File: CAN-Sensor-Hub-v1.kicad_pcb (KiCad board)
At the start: 2 copper layers, 51 x 55 mm, 62 parts, among them J1 Conn_01x04, J10 Conn_01x03, J11 Conn_01x03, J2 Conn_01x04, J3 Conn_01x04, J4 USB_C_Receptacle_USB2.0_14P, J5 Conn_ARM_JTAG_SWD_10, J6 Conn_01x04, J7 Conn_01x04, J8 Conn_01x04, J9 Conn_01x03, Q1 NMOS, Q2 NMOS, Q3 PMOS, SW1 NRST, SW2 BOOT, U1 TPS5430DDA, U2 TCAN1042DRQ1, U3 W25Q32JVZP, U4 AZ1117-3.3, U7 STM32F722VETx, X1 8MHz, X2 32.768KHz

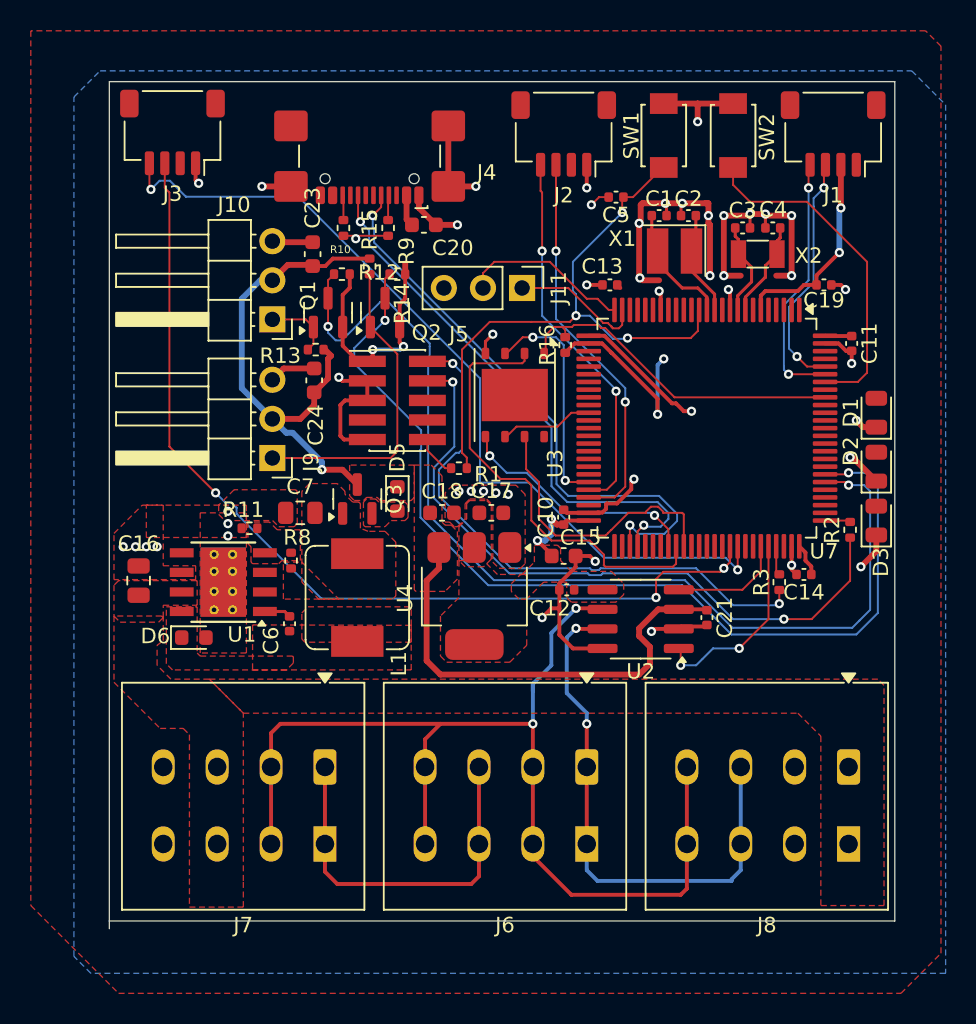
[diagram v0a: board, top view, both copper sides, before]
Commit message: V0.2 of board, nearly ready for production
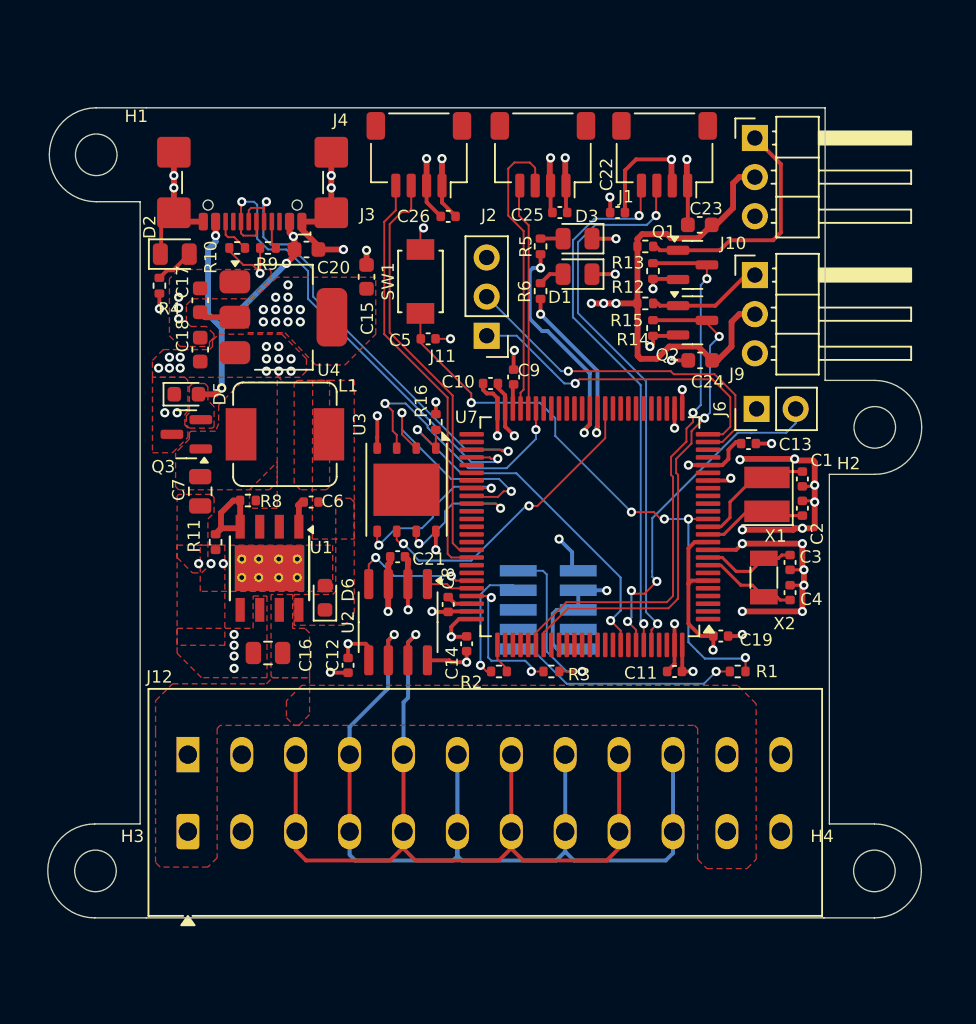
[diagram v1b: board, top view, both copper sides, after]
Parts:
- removed J7, J8: Conn_01x04, TerminalBlock_WAGO:TerminalBlock_WAGO_2601-1104_1x04_P3.50mm_Horizontal
- removed SW2: BOOT, lib:SW_TS-1088-AR02016
- added C22: 100nF, Capacitor_SMD:C_0402_1005Metric, F.Cu at (156.0, 67.5)
- added C25: 100nF, Capacitor_SMD:C_0402_1005Metric, F.Cu at (152.2, 67.5)
- added C26: 100nF, Capacitor_SMD:C_0402_1005Metric, F.Cu at (145.0, 67.8)
- added C8: 2.2uF, Capacitor_SMD:C_0402_1005Metric, F.Cu at (145.0, 93.0)
- added C9: 2.2uF, Capacitor_SMD:C_0402_1005Metric, F.Cu at (149.2, 78.2)
- added H1: MountingHole, MountingHole:MountingHole_2.7mm_M2.5, F.Cu at (122.2, 63.8)
- added H2: MountingHole, MountingHole:MountingHole_2.7mm_M2.5, F.Cu at (172.7, 81.5)
- added H3: MountingHole, MountingHole:MountingHole_2.7mm_M2.5, F.Cu at (122.1, 110.2)
- added H4: MountingHole, MountingHole:MountingHole_2.7mm_M2.5, F.Cu at (172.7, 110.2)
- added J12: Conn_01x12, TerminalBlock_WAGO:TerminalBlock_WAGO_2601-1112_1x12_P3.50mm_Horizontal, F.Cu at (128.1, 107.7)
- added R4: 160, Resistor_SMD:R_0402_1005Metric, F.Cu at (126.2, 72.2)
- added R5: 60, Resistor_SMD:R_0402_1005Metric, F.Cu at (151.0, 69.7)
- added R6: 160, Resistor_SMD:R_0402_1005Metric, F.Cu at (151.0, 72.6)
- J5: moved to B.Cu
- J6: value Conn_01x04 -> Conn_01x02; footprint TerminalBlock_WAGO:TerminalBlock_WAGO_2601-1104_1x04_P3.50mm_Horizontal -> Connector_PinHeader_2.54mm:PinHeader_1x02_P2.54mm_Vertical
- moved D2 47.6 mm to (127.2, 70.2), turned to 0 degrees
- moved J9 33.5 mm to (164.9, 71.6), turned to 0 degrees
- moved J10 33.5 mm to (164.9, 62.7), turned to 0 degrees
- moved D3 26.7 mm to (153.4, 69.2), turned to 180 degrees
- moved J6 25.7 mm to (165.0, 80.2), turned to 90 degrees
- moved C23 25.2 mm to (161.3, 68.3), turned to 180 degrees
- moved C24 25.1 mm to (161.4, 77.1), turned to 180 degrees
- moved R2 24.6 mm to (148.3, 97.3), turned to 0 degrees
- moved C11 24.2 mm to (159.7, 97.3), turned to 180 degrees
- moved Q1 23.9 mm to (160.9, 70.9), turned to 0 degrees
- moved C19 23.8 mm to (162.7, 95.0)
- moved C4 23.7 mm to (167.2, 92.2), turned to 90 degrees
- moved C17 23.4 mm to (128.9, 73.2), turned to 90 degrees
- moved R13 22.4 mm to (157.8, 69.7), turned to 0 degrees
- moved R1 22.4 mm to (163.8, 97.3)
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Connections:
- D1 pad 2: unconnected-(D1-A-Pad2) -> Net-(D1-A)
- D2 pad 2: unconnected-(D2-A-Pad2) -> Net-(D2-A)
- D3 pad 2: unconnected-(D3-A-Pad2) -> Net-(D3-A)
- J11 pad 1: USART2_TX -> USART2_RX
- J11 pad 2: USART2_RX -> USART2_TX
- J6 pad 1: CAN_H -> GNDREF
- J6 pad 2: CAN_L -> Net-(J6-Pin_2)
- U7 pad 37: unconnected-(U7-PE7-Pad37) -> IO_LED3
- U7 pad 38: unconnected-(U7-PE8-Pad38) -> IO_LED2
- U7 pad 39: unconnected-(U7-PE9-Pad39) -> IO_LED1
- U7 pad 48: unconnected-(U7-VCAP_1-Pad48) -> Net-(U7-VCAP_1)
- U7 pad 73: unconnected-(U7-VCAP_2-Pad73) -> Net-(U7-VCAP_2)
- U7 pad 94: Net-(U7-BOOT0) -> Net-(J6-Pin_2)
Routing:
- net Net-(J5-SWCLK/TCK): track 44.1 -> 8.29 mm, vias 2 -> 1
- net I2C3_SDA: track 61.9 -> 26.8 mm, vias 3 -> 0
- net DIO_1_3V3: track 64.2 -> 33.6 mm
- net DIO_0_3V3: track 67.2 -> 36.7 mm
- net I2C3_SCL: track 55.9 -> 27.2 mm, vias 2 -> 0
- net Net-(J5-SWDIO/TMS): track 37.4 -> 11.3 mm, vias 2 -> 1
- net VBUS_5V: track 2.06 -> 27.3 mm, vias 0 -> 4
- net Net-(J6-Pin_2): track 0.00 -> 22.9 mm, vias 0 -> 3
- net Net-(U7-BOOT0): track 22.1 -> 0.00 mm
- net I2C1_SDA: track 15.8 -> 35.9 mm
- net I2C1_SCL: track 16.7 -> 34.9 mm
- net IO_LED2: track 0.00 -> 15.9 mm, vias 0 -> 2
- net USART2_TX: track 8.70 -> 23.1 mm, vias 0 -> 1
- net QSPI_CLK: track 5.98 -> 19.9 mm, vias 0 -> 2
- net QSPI_IO1: track 29.2 -> 15.3 mm, vias 0 -> 2
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- added copper zone on In1.Cu, net GNDREF
- added copper zone on In2.Cu, net VDD_3V3
- added copper zone on In2.Cu, net VDD_5V
- removed copper zone on B.Cu, net GNDREF
- removed copper zone on F.Cu, net Net-(U1-VSENSE)
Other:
- board size 51 x 55 mm -> 56.8 x 52.6 mm
- copper layers 2 -> 4
